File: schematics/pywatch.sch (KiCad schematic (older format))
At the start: 46 parts

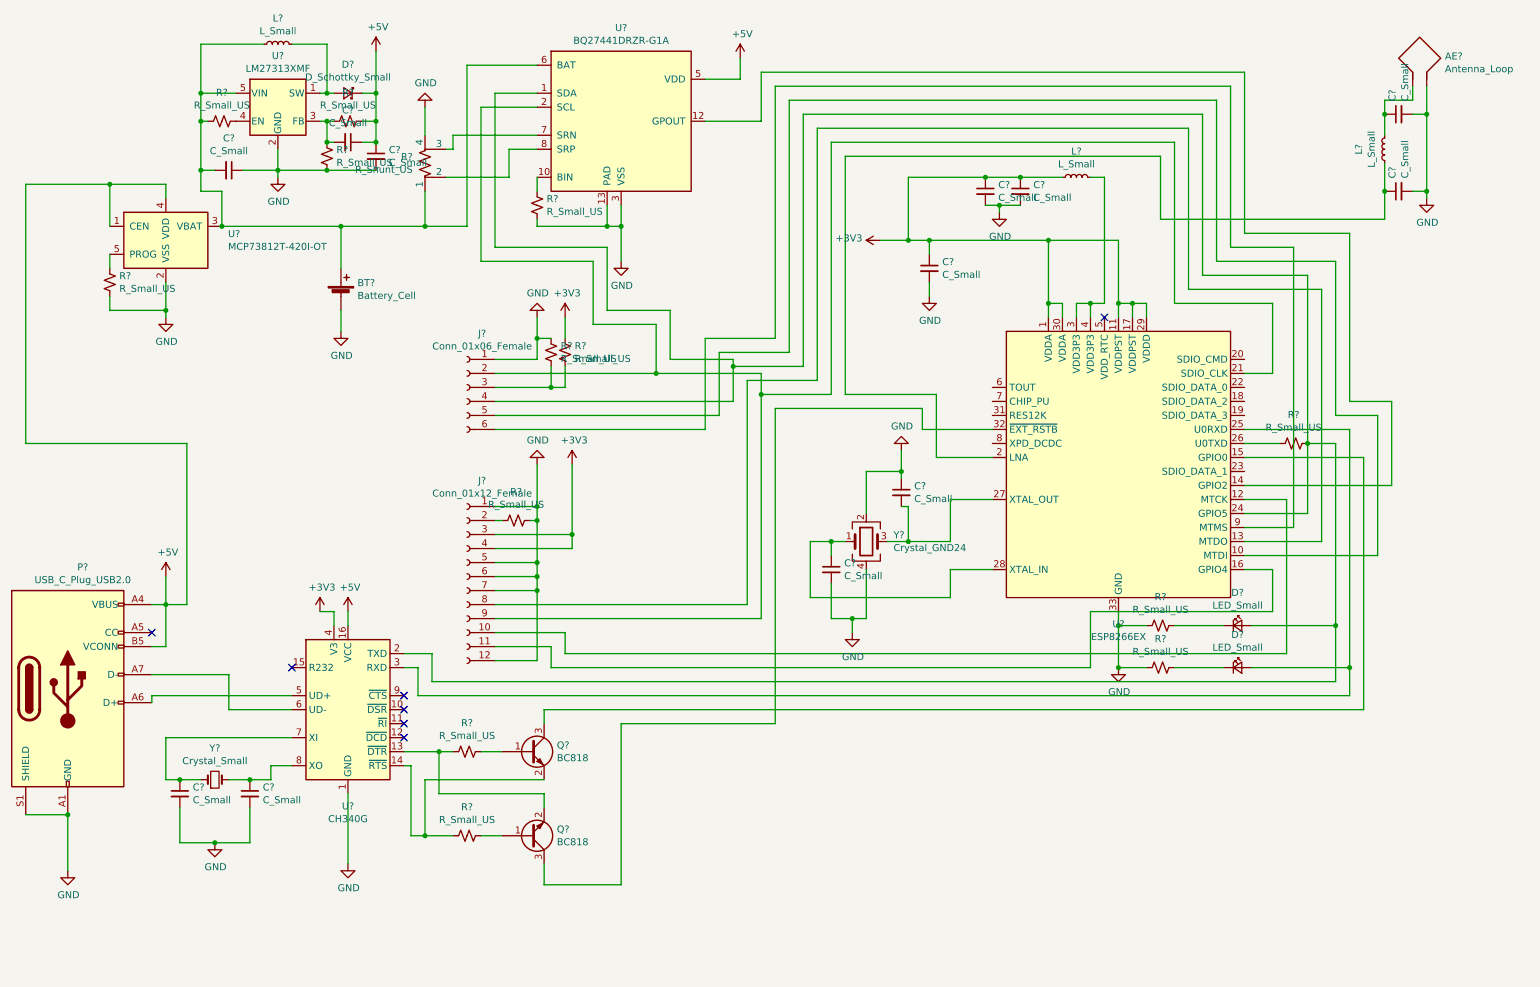
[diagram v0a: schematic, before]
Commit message: completed schematic
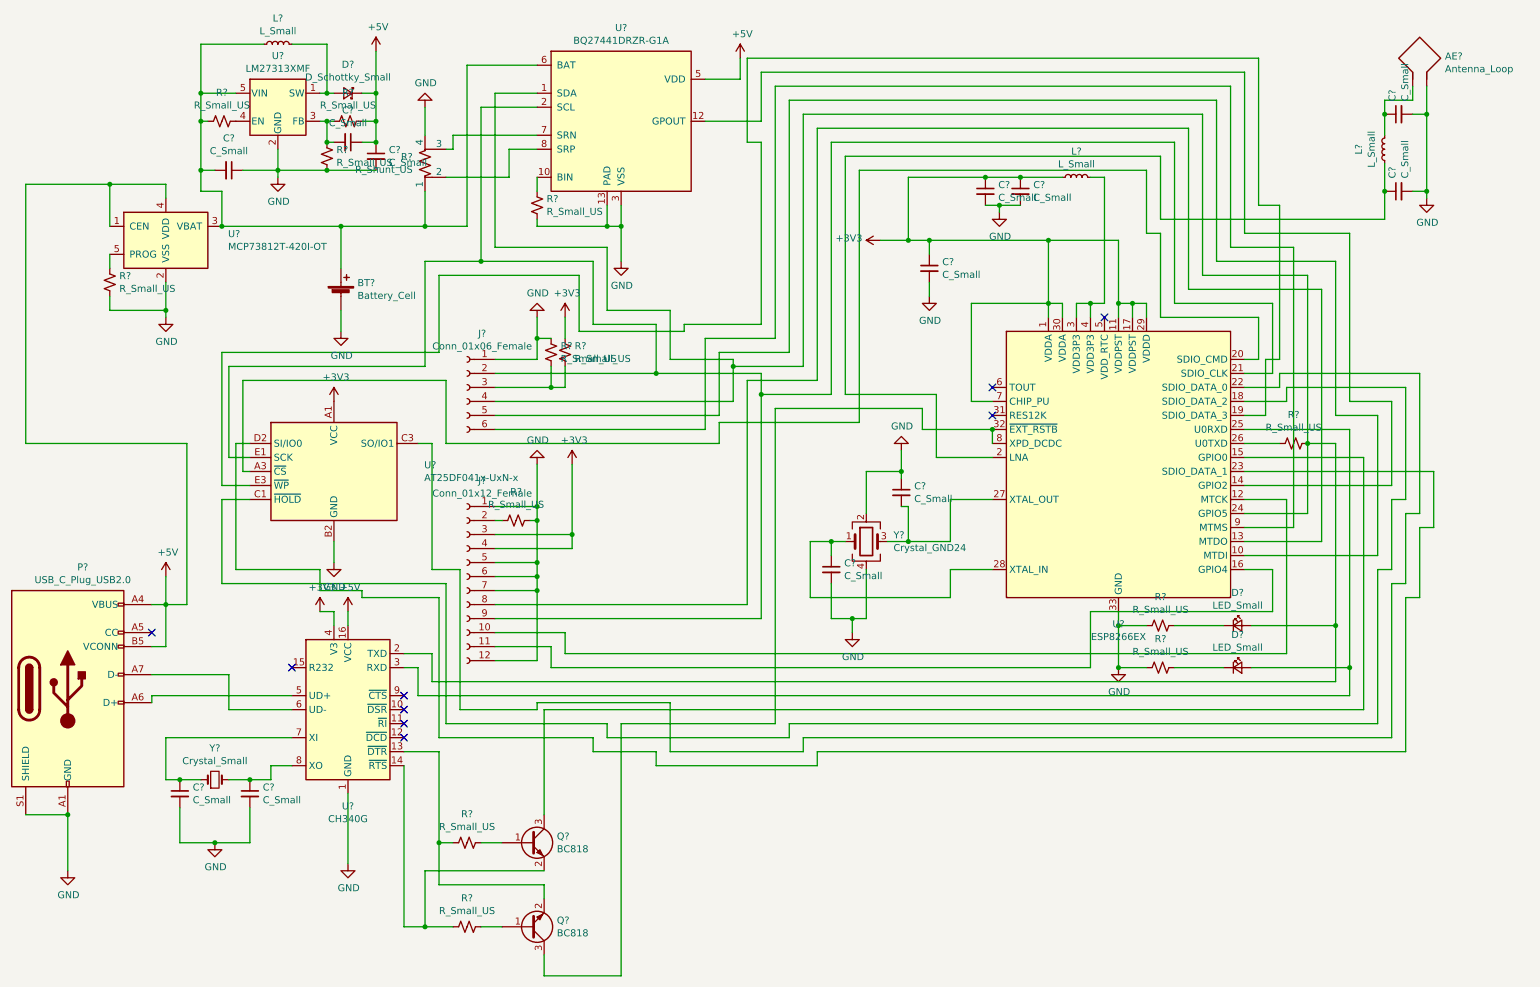
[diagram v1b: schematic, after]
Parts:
- added U?: AT25DF041x-UxN-x, Package_CSP:WLCSP-8_1.58x1.63x0.35mm_Layout3x5_P0.35x0.4mm_Ball0.25mm_Pad0.25mm_NSMD, symbol Memory_Flash:AT25DF041x-UxN-x
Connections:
- net +3V3: now also U?.7 (CHIP_PU), U?.A1 (VCC)
- net GND: now also U?.B2 (GND)
- net at U?.18 (SDIO_DATA_2): now also U?.C1 (~HOLD~)
- net at U?.19 (SDIO_DATA_3): now also U?.E3 (~WP~)
- net at U?.20 (SDIO_CMD): now also U?.A3 (~CS)
- net at J?.2 (Pin_2), J?.9 (Pin_9), U?.2 (SCL)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: now also U?.E1 (SCK)
- net at U?.22 (SDIO_DATA_0): now also U?.C3 (SO/IO1)
- net at U?.23 (SDIO_DATA_1): now also U?.D2 (SI/IO0)
- net at Q?.3 (C), U?.32 (~EXT_RSTB~): now also U?.8 (XPD_DCDC)
- no-connect marks 7 -> 9
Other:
- moved on the sheet: Q?, R?
